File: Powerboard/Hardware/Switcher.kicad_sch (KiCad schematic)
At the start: 40 parts, among them J1 Conn_01x03_MountingPin, J2 Conn_01x02_Male, U1 SN74LVC1G373DCKR, U2 ESP32-S3, Y1 40MHz±10ppm

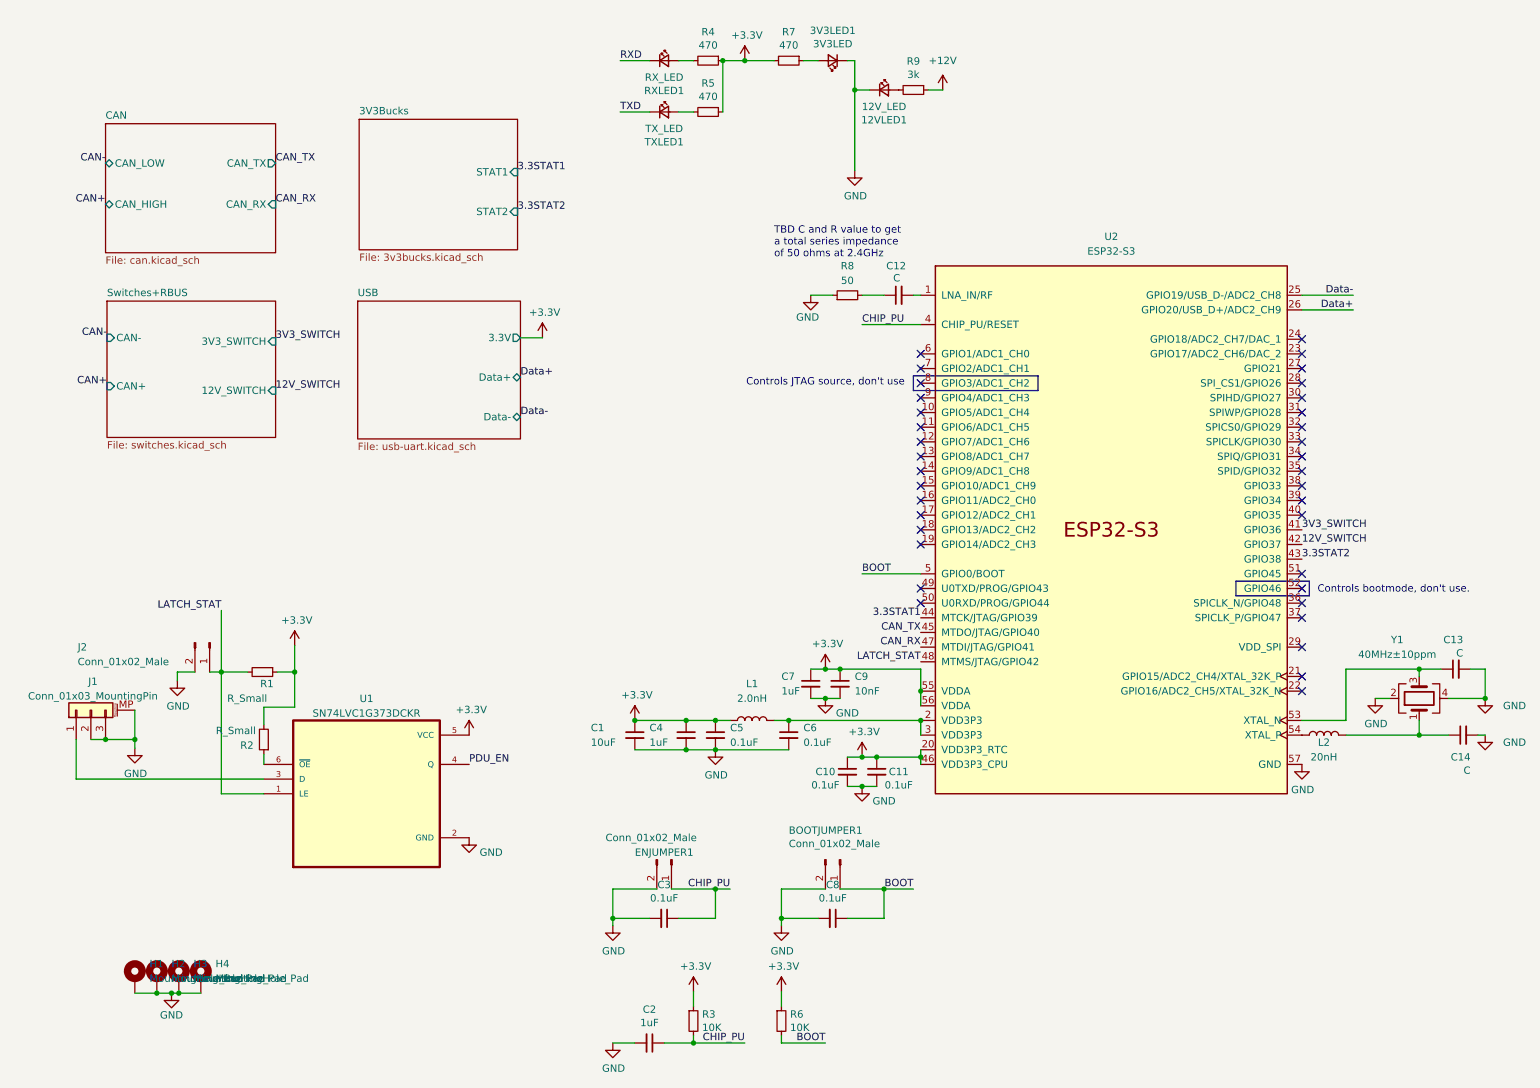
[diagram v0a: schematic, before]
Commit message: latest
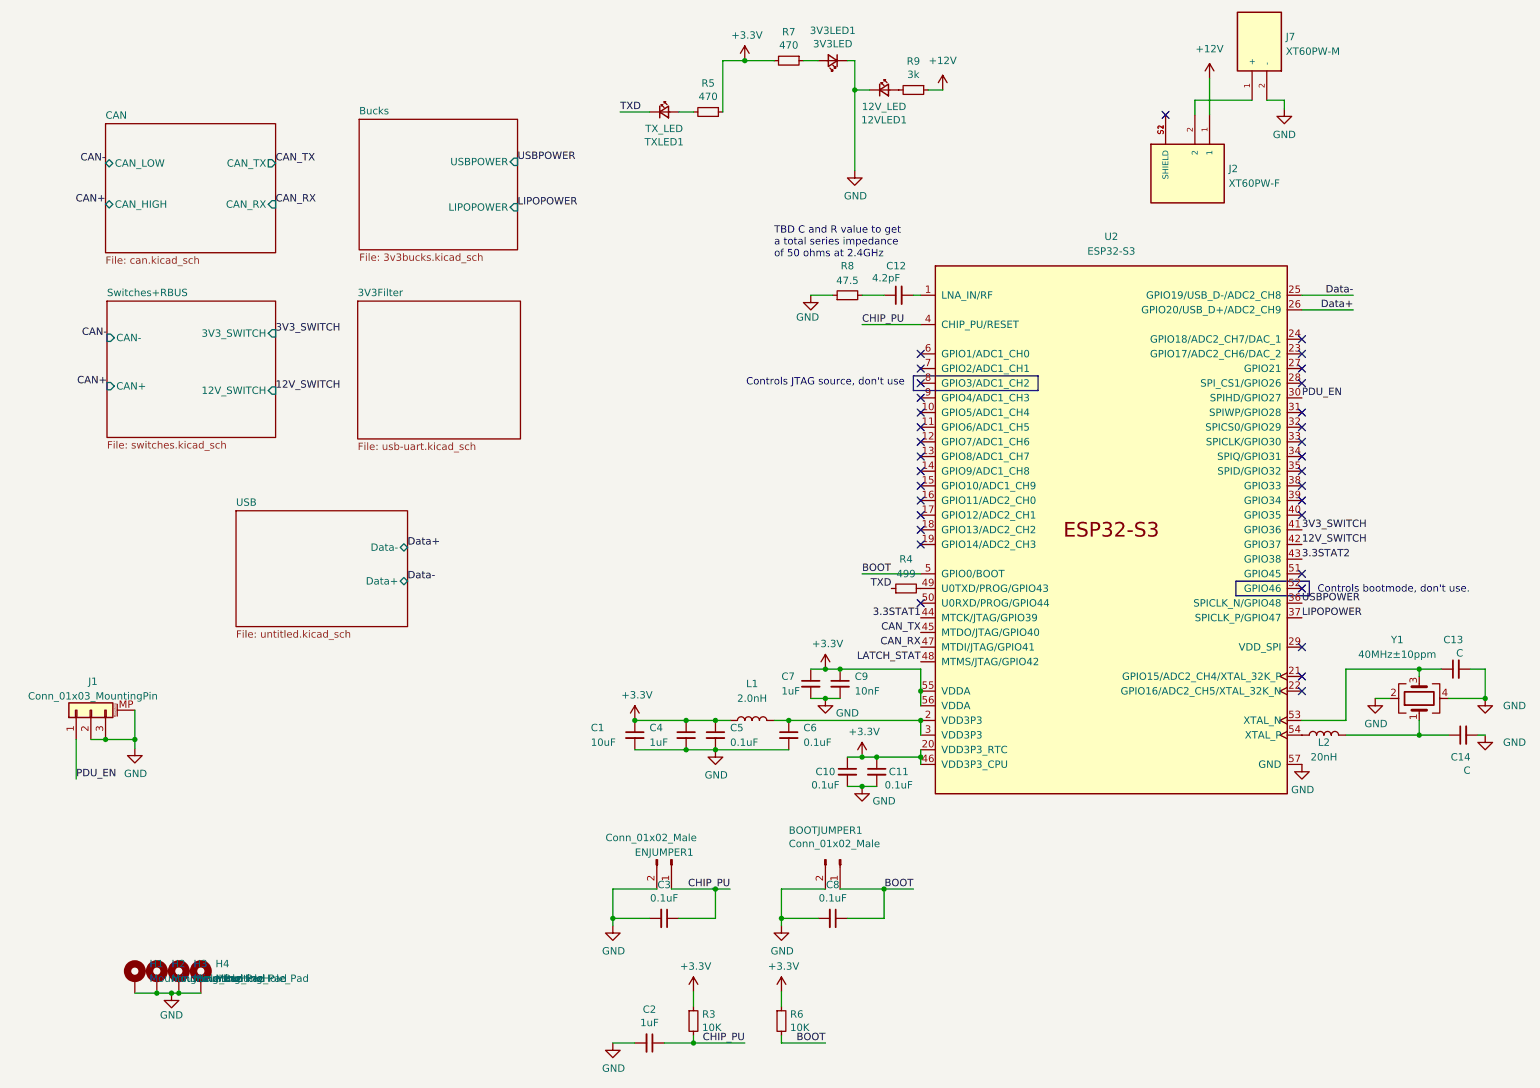
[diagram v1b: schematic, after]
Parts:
- removed J2: Conn_01x02_Male, Connector_Molex:Molex_Nano-Fit_105313-xx02_1x02_P2.50mm_Horizontal, symbol Connector:Conn_01x02_Male
- removed R1, R2: R_Small, Resistor_SMD:R_0402_1005Metric, symbol Device:R_Small
- removed RXLED1: RX_LED, LED_SMD:LED_0603_1608Metric, symbol Device:LED_Small
- removed U1: SN74LVC1G373DCKR, iclr:SOT65P210X110-6N, symbol iclr:SN74LVC1G373DCKR
- added J2: XT60PW-F, iclr:AMASS_XT60PW-F, symbol iclr:XT60PW-F
- added J7: XT60PW-M, iclr:AMASS_XT60PW-M, symbol iclr:XT60PW-M
- C12: value C -> 4.2pF
- R4: value 470 -> 499
- R8: value 50 -> 47.5
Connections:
- net +12V: now also J2.1
- net +3V3: no longer R4.1
- net GND: now also J7.2 (-)
- net PDU_EN: now also J1.1 (Pin_1), U2.30 (SPIHD/GPIO27)
- net TXD: now also R4.1
- net at R4.2: now also U2.49 (U0TXD/PROG/GPIO43)
- net USBPOWER: now reaches U2.36 (SPICLK_N/GPIO48)
- net LIPOPOWER: now reaches U2.37 (SPICLK_P/GPIO47)
- new net: J2.2, J7.1 (+)
- new net: J2.S1 (SHIELD), J2.S2 (SHIELD)
- no-connect marks 36 -> 33
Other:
- sheet 3V3Bucks renamed Bucks
- added sheet 3V3Filter (usb-uart.kicad_sch)
- sheet Bucks ports: added LIPOPOWER, USBPOWER; removed STAT1, STAT2
- sheet USB: file usb-uart.kicad_sch -> untitled.kicad_sch
- sheet USB ports: added none; removed 3.3V
